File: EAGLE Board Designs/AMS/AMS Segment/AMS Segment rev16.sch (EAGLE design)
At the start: 145 parts, among them J0 CONNECTOR-1_5222_, J1 CONNECTOR-1_5222_, J10 CONNECTOR-1_5222_, J11 CONNECTOR-1_5222_, J12 CONNECTOR-1_5222_, J13 CONNECTOR-1_5222_, J14 CONNECTOR-1_5222_, J15 CONNECTOR-1_5222_, J16 CONNECTOR-1_5222_, J17 CONNECTOR-1_5222_, J18 CONNECTOR-1_5222_, J2 CONNECTOR-1_5222_, J27 CONNECTOR-2_MICROFIT_SMD_RIGH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, J28 CONNECTOR-2_MICROFIT_SMD_RIGH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, J29 CONNECTOR-1_5222_, J3 CONNECTOR-1_5222_, J30 CONNECTOR-1_5222_, J31 CONNECTOR-1_5222_, J32 CONNECTOR-2_MICROFIT_SMD_RIGH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, J33 CONNECTOR-2_MICROFIT_SMD_RIGH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, J34 CONNECTOR-2_MICROFIT_SMD_RIGH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, J35 CONNECTOR-2_MICROFIT_SMD_RIGH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, J37 CONNECTOR-2_MICROFIT_SMD_RIGH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, J38 CONNECTOR-2_MICROFIT_SMD_RIGH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, J39 CONNECTOR-2_MICROFIT_SMD_RIGH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, J4 CONNECTOR-1_5222_, J40 CONNECTOR-2_MICROFIT_SMD_RIGH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, J5 CONNECTOR-1_5222_, J6 CONNECTOR-1_5222_, J7 CONNECTOR-1_5222_, J8 CONNECTOR-1_5222_, J9 CONNECTOR-1_5222_, Q1 TRANSISTOR_NPN, Q2 TRANSISTOR_NPN, T1 TRANSFORMER_HM2112ZNLT, U1 LTC6811-2, U2 LTC6811-2, U3 SHT31-ARP-B, U4 SHT31-ARP-B

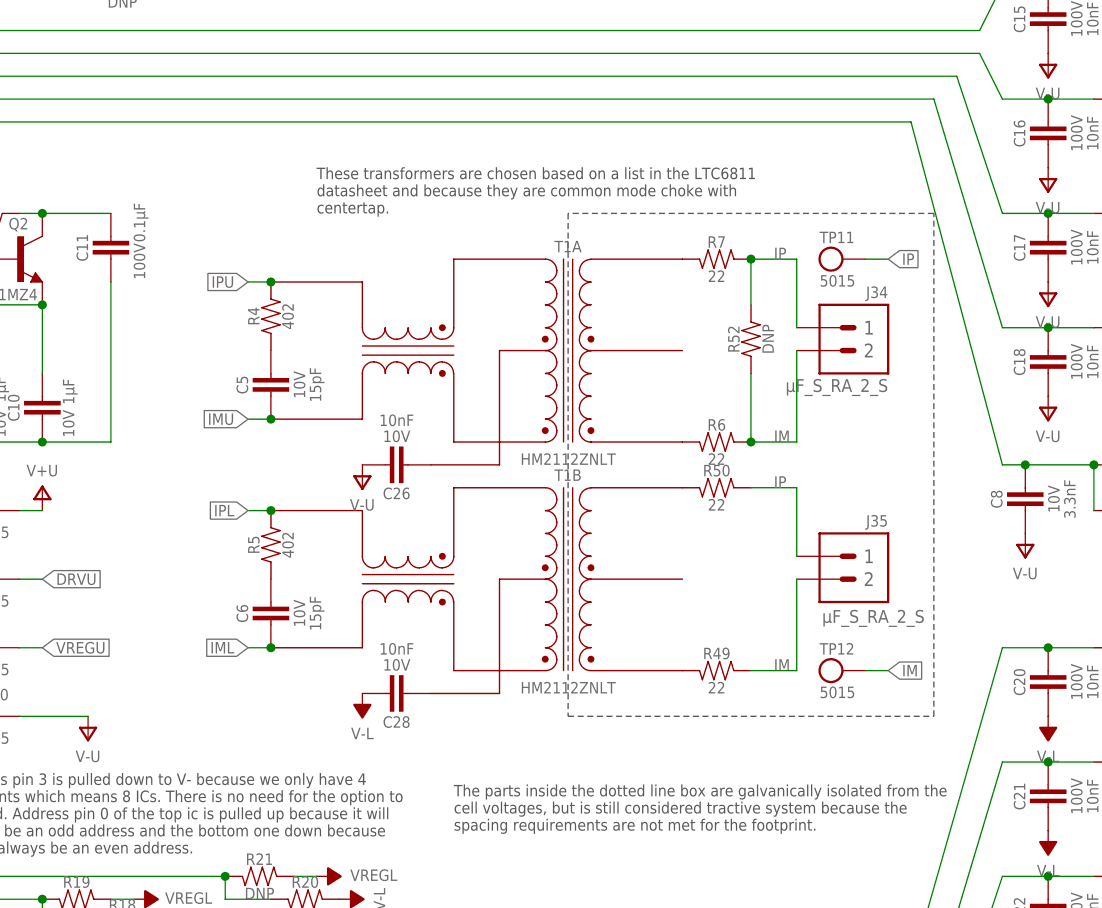
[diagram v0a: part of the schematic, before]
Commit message: AMS schematic approved
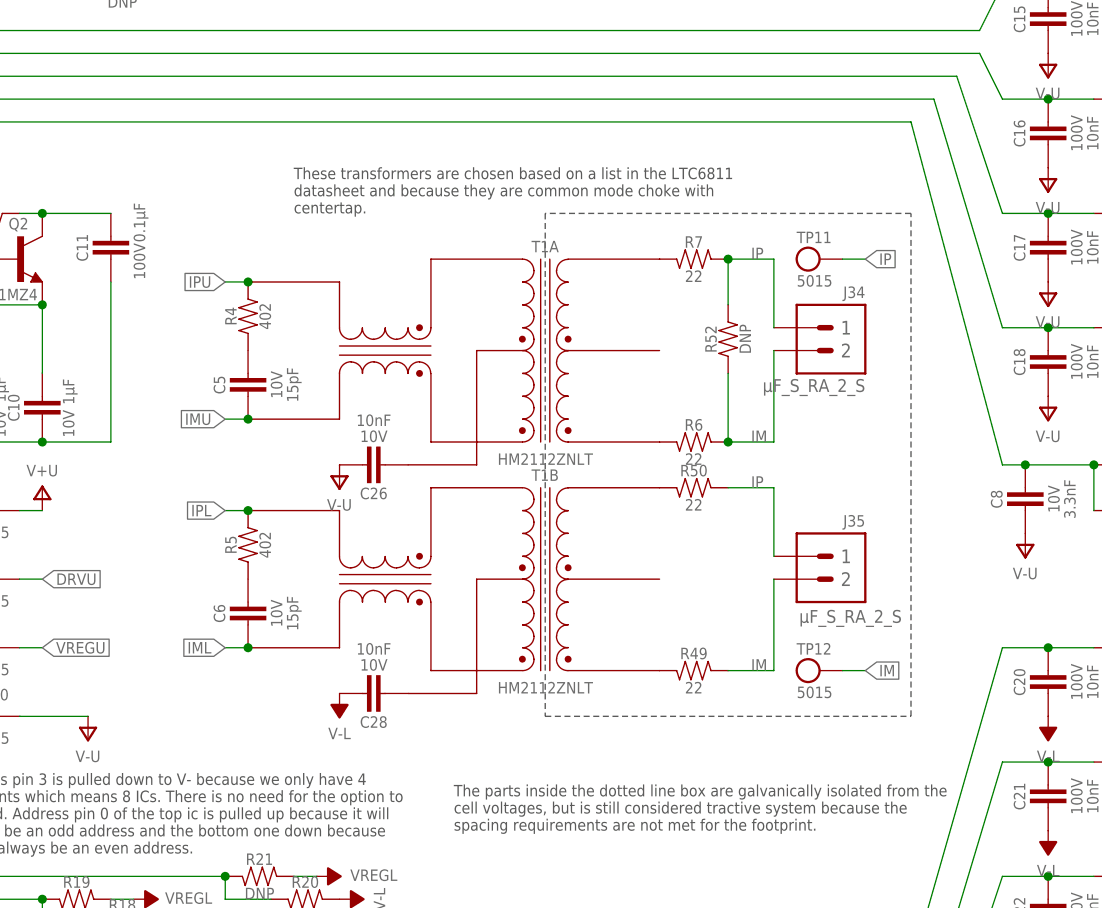
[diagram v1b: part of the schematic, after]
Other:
- moved on the sheet: C26, C28, C5, C6, J34, J35, R4, R49, R5, R50, R52, R6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
